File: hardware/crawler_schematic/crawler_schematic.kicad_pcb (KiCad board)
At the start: 4 copper layers, 112 x 72 mm, 31 parts, among them J2 JST-PH, J4 JST-PH, M2 Motor_Servo, Q1 AO4407A, U1 NRF24L01, U2 TB6612FNG, U5 RY8336

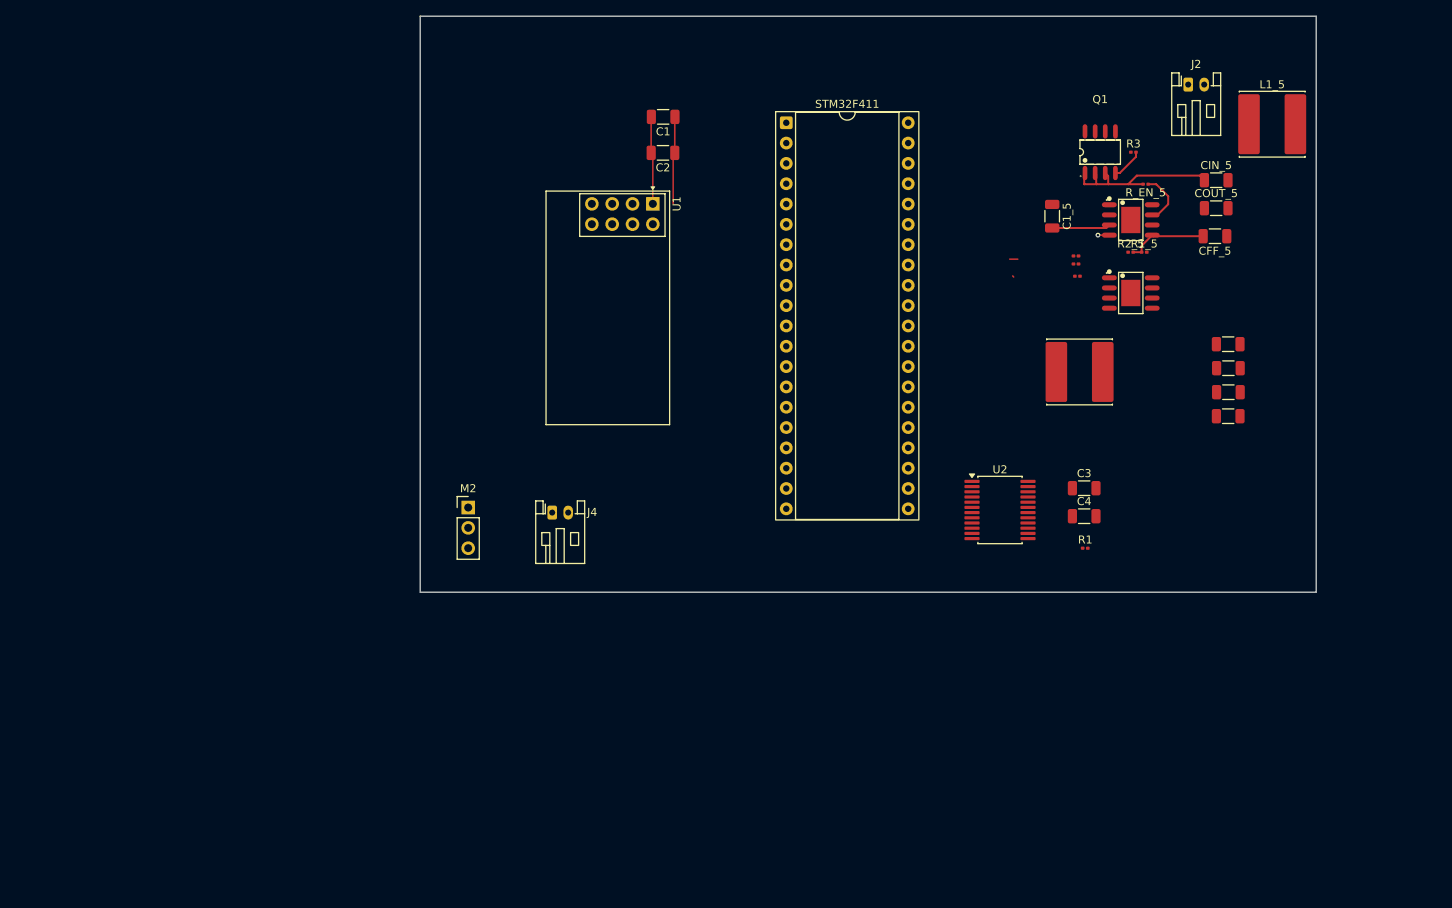
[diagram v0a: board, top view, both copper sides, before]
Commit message: update: pcb work, power layers
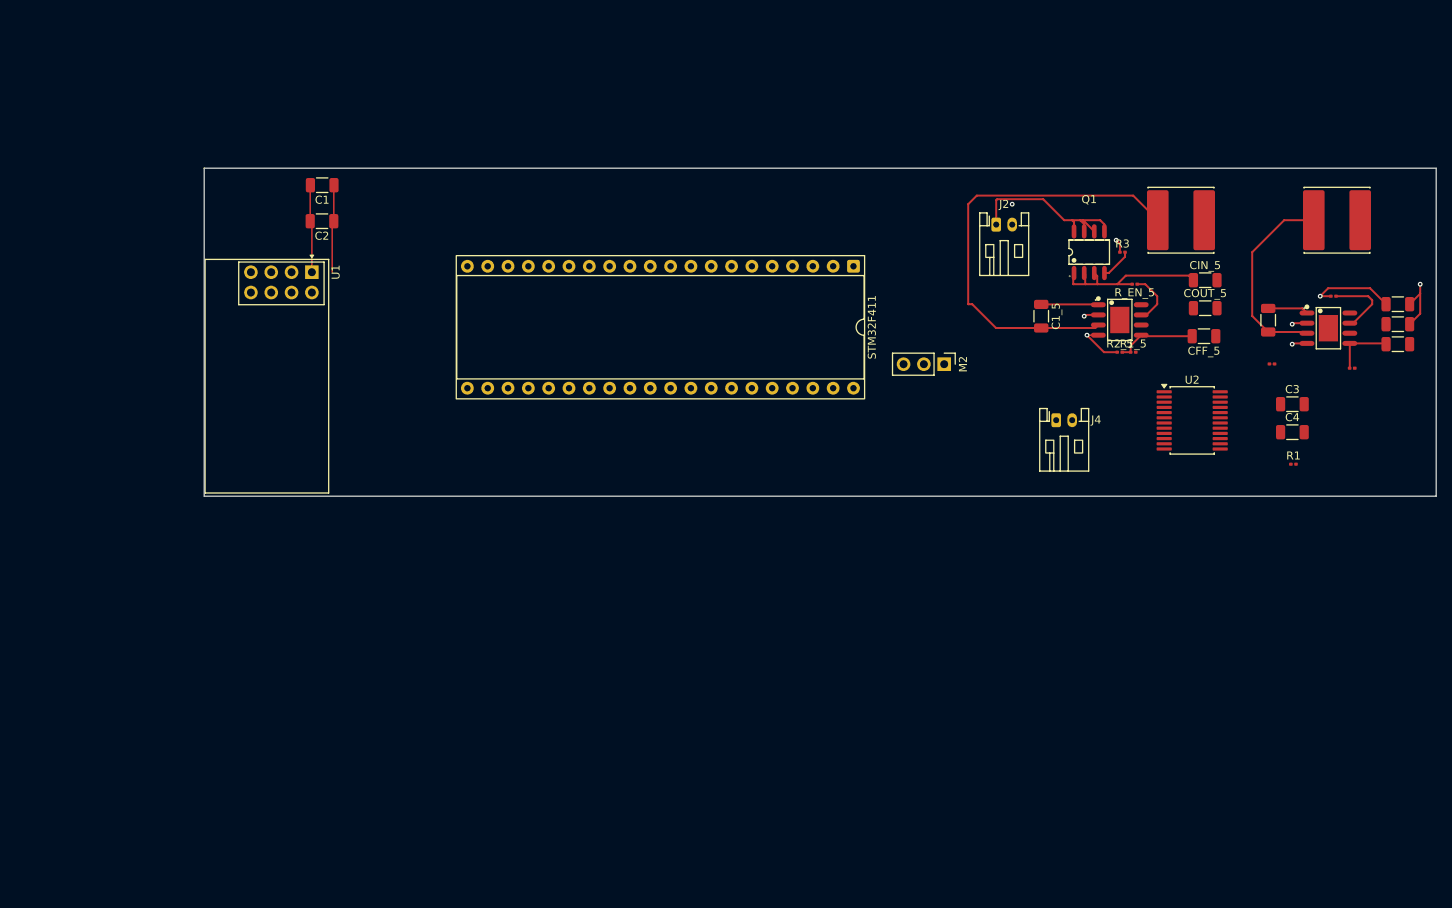
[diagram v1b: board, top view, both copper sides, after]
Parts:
- moved J4 64.0 mm to (230.0, 91.0)
- moved M2 62.1 mm to (216.0, 84.0), turned to -90 degrees
- moved C2 43.5 mm to (138.2, 66.1)
- moved U1 43.5 mm to (137.0, 72.5)
- moved C1 43.5 mm to (138.2, 61.6)
- moved L1_3.3 37.4 mm to (265.1, 66.0)
- moved R1_3.3 37.3 mm to (267.0, 84.5)
- moved R_EN_3.3 32.1 mm to (264.7, 75.5), turned to 180 degrees
- moved J2 29.7 mm to (222.5, 66.5)
- moved C3 28.1 mm to (259.5, 89.0)
- moved C4 28.1 mm to (259.5, 92.5)
- moved R1 28.1 mm to (259.7, 96.5)
- moved R2_3.3 27.5 mm to (257.0, 84.0)
- moved U2 26.5 mm to (247.0, 91.0)
- moved U_3.3 25.1 mm to (264.0, 79.5)
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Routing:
- net Net-(U5-SW): track 7.30 -> 55.6 mm
- net Net-(U_3.3-SW): track 0.00 -> 25.1 mm
- net Net-(J2-Pin_1): track 0.00 -> 23.9 mm
- net GND: track 12.4 -> 30.6 mm, vias 1 -> 5
- net +BATT: track 22.2 -> 36.6 mm, vias 0 -> 3
- net Net-(U_3.3-EN): track 0.00 -> 9.01 mm
- net Net-(U_3.3-FB): track 0.00 -> 7.68 mm
- net Net-(U5-BS): track 0.16 -> 7.26 mm
- net Net-(U_3.3-BS): track 0.00 -> 5.08 mm
- net (no net): track 1.00 -> 0.00 mm
- added copper zone on In2.Cu, net +3.3V
- added copper zone on In2.Cu, net +5V
- added copper zone on In2.Cu, net +BATT
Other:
- board size 112 x 72 mm -> 154 x 41 mm

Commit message: update: MITE completion 80%
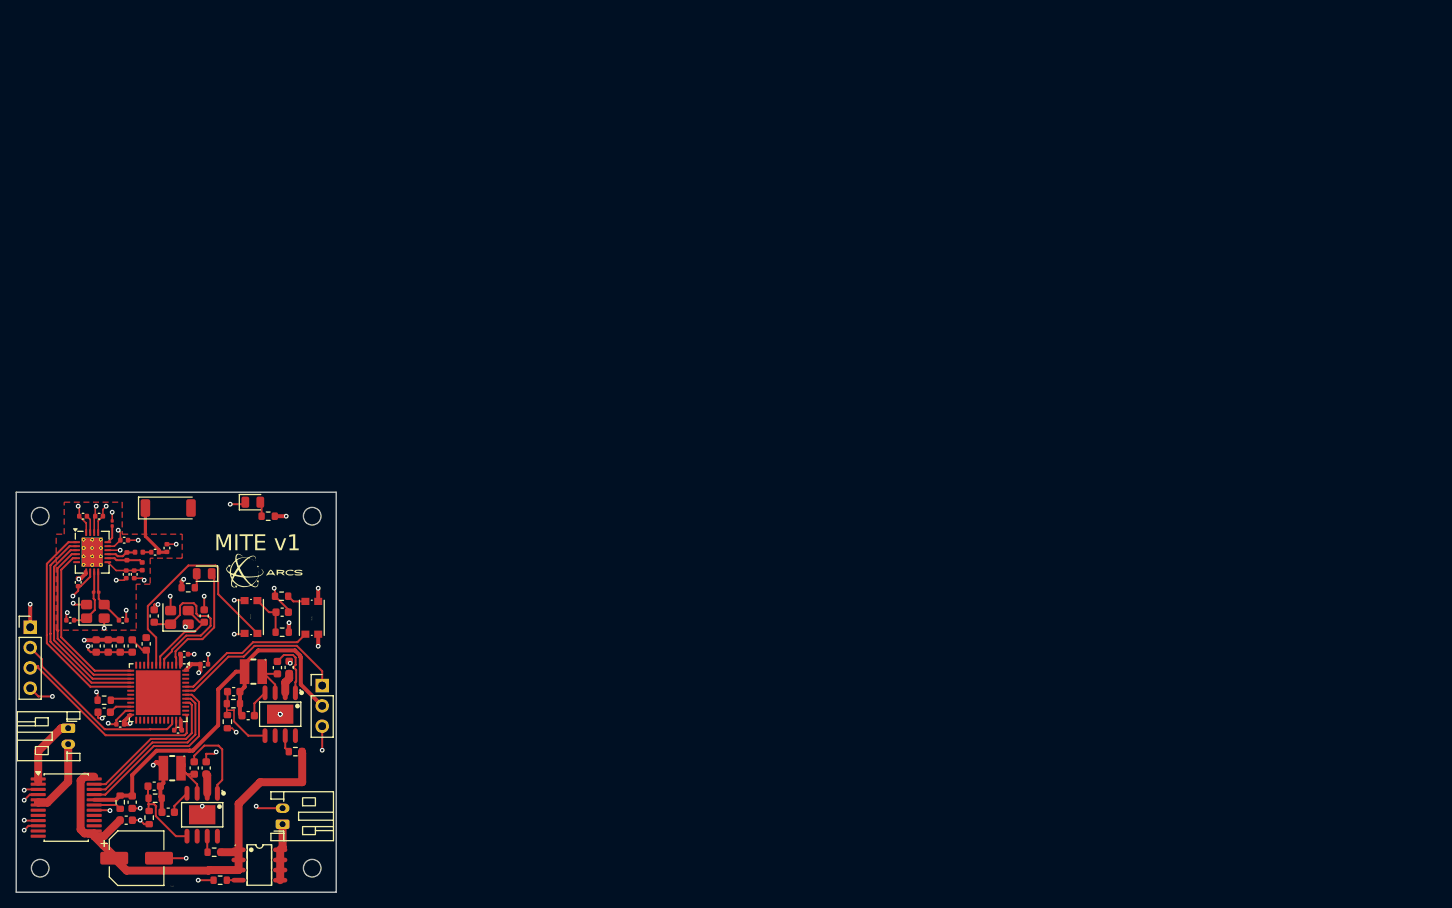
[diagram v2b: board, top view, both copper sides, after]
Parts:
- removed C1, C3, C4: 10uF, Capacitor_SMD:C_1206_3216Metric
- removed C2: 104nF, Capacitor_SMD:C_1206_3216Metric
- removed J4: JST-PH, Connector_JST:JST_PH_S2B-PH-K_1x02_P2.00mm_Horizontal
- removed R1: 10k Ohm, Resistor_SMD:R_0201_0603Metric
- removed R3: 10 kOhm, Resistor_SMD:R_0201_0603Metric
- removed STM32F411: STM32F411_BlackPill, Package_DIP:DIP-40_W15.24mm_Socket
- removed U5, U_3.3: RY8336, easyeda2kicad:ESOP-8_L4.9-W3.9-P1.27-LS6.0-BL-EP-1
- added AE1: 50ohm, RF_Antenna:Johanson_2450AT43F0100, F.Cu at (119.0, 102.0)
- added C_H_1: 10uF, Capacitor_SMD:C_0603_1608Metric, F.Cu at (114.5, 138.8)
- added C_H_2: 10uF, Capacitor_SMD:C_0603_1608Metric, F.Cu at (113.8, 141.0)
- added C_H_3: 47uF, Capacitor_SMD:CP_Elec_6.3x5.4, F.Cu at (115.0, 145.8)
- added C_M_1: 4.3pF, Capacitor_SMD:C_0603_1608Metric, F.Cu at (117.2, 115.5)
- added C_M_2: 4.3pF, Capacitor_SMD:C_0603_1608Metric, F.Cu at (123.5, 115.5)
- added C_M_3: 2.2uF, Capacitor_SMD:C_0603_1608Metric, F.Cu at (111.0, 127.5)
- added C_M_4: 100 nF, X7R, 16 V, Capacitor_SMD:C_0402_1005Metric, F.Cu at (123.5, 121.5)
- added C_M_5: 100 nF, X7R, 16 V, Capacitor_SMD:C_0402_1005Metric, F.Cu at (120.2, 129.8)
- added C_M_6: 100 nF, X7R, 16 V, Capacitor_SMD:C_0402_1005Metric, F.Cu at (113.0, 129.0)
- added C_M_7: 100 nF, X7R, Capacitor_SMD:C_0402_1005Metric, F.Cu at (121.0, 120.2)
- added C_nrf_1: 10nF, Capacitor_SMD:C_0402_1005Metric, F.Cu at (110.4, 103.0)
- added C_nrf_11: 10nF, Capacitor_SMD:C_0402_1005Metric, F.Cu at (107.8, 111.3)
- added C_nrf_2: 1nF, Capacitor_SMD:C_0402_1005Metric, F.Cu at (113.5, 106.0)
- added C_nrf_3: 33nF, Capacitor_SMD:C_0402_1005Metric, F.Cu at (108.4, 103.0)
- added C_nrf_4: 1.0pF, Capacitor_SMD:C_0402_1005Metric, F.Cu at (118.8, 107.0)
- added C_nrf_5: 1.5pF, Capacitor_SMD:C_0402_1005Metric, F.Cu at (117.4, 107.5)
- added C_nrf_6: 4.7pF, Capacitor_SMD:C_0402_1005Metric, F.Cu at (113.8, 110.3)
- added C_nrf_7: 2.2nF, Capacitor_SMD:C_0402_1005Metric, F.Cu at (114.8, 110.3)
- added C_nrf_8: 22pF, Capacitor_SMD:C_0402_1005Metric, F.Cu at (106.8, 116.0)
- added C_nrf_9: 22pF, Capacitor_SMD:C_0402_1005Metric, F.Cu at (113.3, 116.0)
- added C_ref_1: Opt., Capacitor_SMD:C_0603_1608Metric, F.Cu at (110.0, 119.2)
- added C_ref_2: Opt., Capacitor_SMD:C_0603_1608Metric, F.Cu at (111.5, 119.2)
- added C_ref_3: Opt., Capacitor_SMD:C_0603_1608Metric, F.Cu at (113.0, 119.2)
- added C_ref_4: Opt., Capacitor_SMD:C_0603_1608Metric, F.Cu at (114.5, 119.2)
- added C_rst_1: 100nF, Capacitor_SMD:C_0603_1608Metric, F.Cu at (133.2, 115.0)
- added D_L_1: LED_pc13, LED_SMD:LED_0805_2012Metric, F.Cu at (123.5, 110.2)
- added D_L_2: LED_pwr, LED_SMD:LED_0805_2012Metric, F.Cu at (129.6, 101.2)
- added G***: LOGO, footprints:arcs_medium_logo, F.Cu at (131.2, 109.8)
- added J1: JST-PH, Connector_JST:JST_PH_S2B-PH-K_1x02_P2.00mm_Horizontal, F.Cu at (133.3, 141.5)
- added J3: SWD_Header, Connector_PinHeader_2.54mm:PinHeader_1x04_P2.54mm_Vertical, F.Cu at (101.8, 116.9)
- added L_M_1: 10uH +-10%, Inductor_SMD:L_0603_1608Metric, F.Cu at (116.2, 119.0)
- added L_nrf_1: 8.2nH, Inductor_SMD:L_0402_1005Metric, F.Cu at (113.8, 108.0)
- added L_nrf_2: 3.9nH, Inductor_SMD:L_0402_1005Metric, F.Cu at (115.3, 107.5)
- added L_nrf_3: 2.7nH, Inductor_SMD:L_0402_1005Metric, F.Cu at (115.8, 109.3)
- added R3_5: 10 kOhm, Resistor_SMD:R_0603_1608Metric, F.Cu at (126.4, 128.7)
- added REF**: MountingHole_2.2mm_M2, MountingHole:MountingHole_2.2mm_M2, F.Cu at (137.0, 147.0)
- added REF**: MountingHole_2.2mm_M2, MountingHole:MountingHole_2.2mm_M2, F.Cu at (103.0, 103.0)
- added REF**: MountingHole_2.2mm_M2, MountingHole:MountingHole_2.2mm_M2, F.Cu at (137.0, 103.0)
- added REF**: MountingHole_2.2mm_M2, MountingHole:MountingHole_2.2mm_M2, F.Cu at (103.0, 147.0)
- added R_B_1: 10K, Resistor_SMD:R_0603_1608Metric, F.Cu at (133.2, 113.0)
- added R_B_2: 10K, Resistor_SMD:R_0603_1608Metric, F.Cu at (111.0, 126.0)
- added R_H_1: 10k Ohm, Resistor_SMD:R_0603_1608Metric, F.Cu at (113.0, 138.8)
- added R_L_1: 1K, Resistor_SMD:R_0603_1608Metric, F.Cu at (121.5, 111.9)
- added R_L_2: 5.1K, Resistor_SMD:R_0603_1608Metric, F.Cu at (131.5, 103.0)
- added R_nrf_1: 22k, Resistor_SMD:R_0201_0603Metric, F.Cu at (112.0, 103.9)
- added R_nrf_2: 1M, Resistor_SMD:R_0201_0603Metric, F.Cu at (110.0, 112.5)
- added R_rst_1: NC, Resistor_SMD:R_0603_1608Metric, F.Cu at (133.2, 117.5)
- added SW_B_1: boot switch, Button_Switch_SMD:SW_Push_1P1T_NO_CK_KMR2, F.Cu at (136.9, 115.7)
- added SW_rst_2: nrst_switch, Button_Switch_SMD:SW_Push_1P1T_NO_CK_KMR2, F.Cu at (129.3, 115.6)
- added U3: RY8336, easyeda2kicad:ESOP-8_L4.9-W3.9-P1.27-LS6.0-BL-EP-1, F.Cu at (123.2, 140.3)
- added U4: TB6612FNG, Package_SO:SSOP-24_5.3x8.2mm_P0.65mm, F.Cu at (106.2, 139.4)
- added U6: NRF24L01, Package_DFN_QFN:QFN-20-1EP_4x5mm_P0.5mm_EP2.65x3.65mm_ThermalVias, F.Cu at (109.5, 107.5)
- added Y_M_1: Crystal_4pin_GND24, Crystal:Crystal_SMD_3225-4Pin_3.2x2.5mm, F.Cu at (120.4, 115.7)
- added Y_nrf_1: Crystal_4pin_GND24, Crystal:Crystal_SMD_3225-4Pin_3.2x2.5mm, F.Cu at (109.9, 114.9)
- C1_3.3, C1_5, CFF_3.3, CFF_5, CIN_3.3, CIN_5, COUT_3.3, COUT_5: footprint Capacitor_SMD:C_1206_3216Metric -> Capacitor_SMD:C_0603_1608Metric
- L1_3.3, L1_5: footprint Inductor_SMD:L_Cenker_CKCS8040 -> easyeda2kicad:IND-SMD_L3.0-W3.0_FTC303020D
- R1_3.3, R2_3.3, R_EN_3.3, R_EN_5: footprint Resistor_SMD:R_0201_0603Metric -> Resistor_SMD:R_0603_1608Metric
- R1_5: value 44.05 kOhm -> 10 kOhm; footprint Resistor_SMD:R_0201_0603Metric -> Resistor_SMD:R_0603_1608Metric
- R2_5: value 10 kOhm -> 44.05 kOhm; footprint Resistor_SMD:R_0201_0603Metric -> Resistor_SMD:R_0603_1608Metric
- U1: value NRF24L01 -> STM32F411CEUx; footprint RF_Module:nRF24L01_Breakout -> Package_DFN_QFN:QFN-48-1EP_7x7mm_P0.5mm_EP5.6x5.6mm
- U2: value TB6612FNG -> RY8336; footprint Package_SO:SSOP-24_5.3x8.2mm_P0.65mm -> easyeda2kicad:ESOP-8_L4.9-W3.9-P1.27-LS6.0-BL-EP-1
- moved COUT_3.3 165.4 mm to (119.0, 140.0)
- moved CFF_3.3 165.0 mm to (117.2, 136.8)
- moved L1_3.3 160.9 mm to (119.5, 134.5), turned to 180 degrees
- moved CIN_3.3 159.8 mm to (123.8, 134.5), turned to 90 degrees
- moved R1_3.3 159.0 mm to (117.4, 138.2)
- moved R_EN_3.3 156.2 mm to (124.8, 145.0), turned to 0 degrees
- moved R2_3.3 151.4 mm to (116.6, 140.7), turned to 90 degrees
- moved C1_3.3 145.5 mm to (122.2, 134.5)
- moved J2 132.0 mm to (106.5, 129.5), turned to -90 degrees
- moved R1_5 131.8 mm to (125.5, 148.5)
- moved COUT_5 130.0 mm to (129.0, 127.9)
- moved CFF_5 129.2 mm to (127.2, 124.9)
- moved L1_5 129.0 mm to (129.7, 122.4), turned to 180 degrees
- moved Q1 128.9 mm to (130.4, 146.6), turned to -90 degrees
- moved CIN_5 124.3 mm to (134.1, 121.9), turned to 90 degrees
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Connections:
- C1_5 pad 1: Net-(U5-BS) -> Net-(U2-BS)
- C1_5 pad 2: Net-(U5-SW) -> Net-(U2-SW)
- CFF_5 pad 2: Net-(U5-FB) -> Net-(U2-FB)
- J2 pad 1: Net-(J2-Pin_1) -> AO1
- J2 pad 2: GND -> AO2
- L1_5 pad 1: Net-(U5-SW) -> Net-(U2-SW)
- M2 pad 1: Net-(M2-PWM) -> servo_pwm
- Q1 pad 5: Net-(J2-Pin_1) -> BAT_IN
- Q1 pad 6: Net-(J2-Pin_1) -> BAT_IN
- Q1 pad 7: Net-(J2-Pin_1) -> BAT_IN
- Q1 pad 8: Net-(J2-Pin_1) -> BAT_IN
- R1_5 pad 1: Net-(U5-FB) -> GND
- R1_5 pad 2: +5V -> Net-(Q1-G)
- R2_5 pad 1: GND -> Net-(U2-FB)
- R2_5 pad 2: Net-(U5-FB) -> +5V
- R_EN_5 pad 1: Net-(U5-EN) -> Net-(U2-EN)
- U1 pad 1: GND -> +3.3V
- U1 pad 2: +3.3V -> /PC13
- U1 pad 4: Net-(STM32F411-Pin_30) -> unconnected-(U1-PC15-Pad4)
- U1 pad 7: Net-(STM32F411-Pin_32) -> NRST
- U1 pad 8: Net-(STM32F411-Pin_29) -> GND
- U2 pad 1: Net-(J4-Pin_1) -> Net-(U2-BS)
- U2 pad 2: Net-(J4-Pin_1) -> +BATT
- U2 pad 3: GND -> Net-(U2-SW)
- U2 pad 5: Net-(J4-Pin_2) -> Net-(U2-FB)
- U2 pad 6: Net-(J4-Pin_2) -> unconnected-(U2-NC-Pad6)
- U2 pad 7: unconnected-(U2-BO2-Pad7)_1 -> Net-(U2-EN)
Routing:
- net GND: track 30.6 -> 92.1 mm, vias 5 -> 45
- net Net-(U5-SW): track 55.6 -> 0.00 mm
- net +5V: track 0.00 -> 52.6 mm
- net NRST: track 0.00 -> 35.0 mm
- net CE: track 0.00 -> 27.5 mm
- net +3.3V: track 11.0 -> 37.8 mm, vias 0 -> 13
- net +BATT: track 36.6 -> 62.9 mm, vias 3 -> 0
- net ~{CSN}: track 0.00 -> 26.0 mm
- net /PA14: track 0.00 -> 25.8 mm
- net SCK: track 0.00 -> 24.4 mm
- net Net-(J2-Pin_1): track 23.9 -> 0.00 mm
- net /PA13: track 0.00 -> 23.3 mm
- net MOSI: track 0.00 -> 22.9 mm
- net servo_pwm: track 0.00 -> 22.5 mm
- net AIN1: track 0.00 -> 22.4 mm
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- added copper zone on F.Cu, net GND
- removed copper zone on In2.Cu, net +5V
- removed copper zone on In2.Cu, net +BATT
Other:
- board size 154 x 41 mm -> 40 x 50 mm
- board text added: "MITE v1"
